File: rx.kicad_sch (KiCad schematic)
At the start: 1 part, among them U1 CC1200

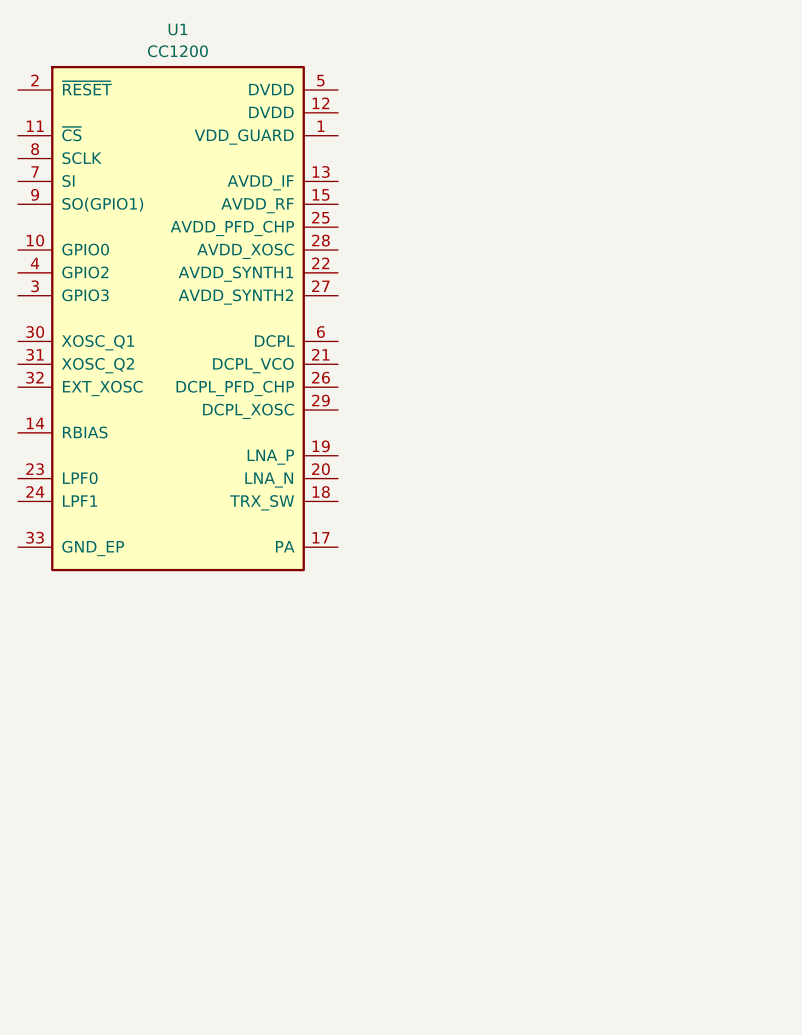
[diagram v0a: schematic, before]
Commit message: Add files via upload
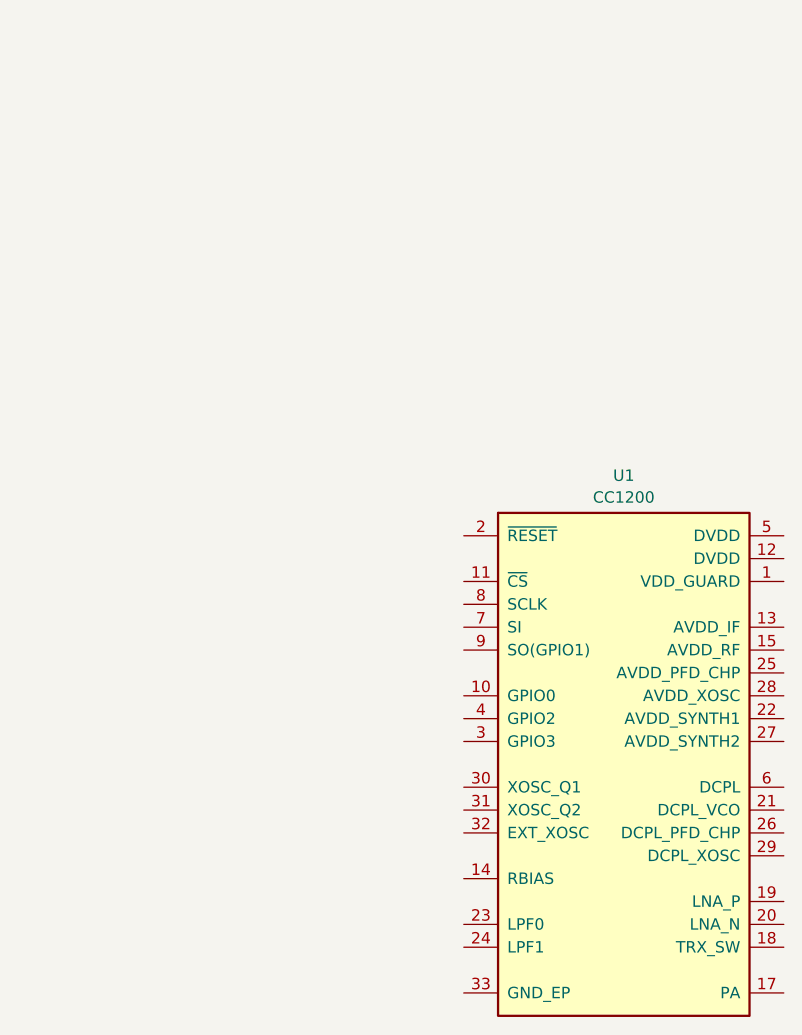
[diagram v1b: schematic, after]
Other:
- moved on the sheet: U1
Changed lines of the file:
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@@
     (comment 1 "Wojciech Kaczmarski, SP5WWP")
   )
-  (symbol (lib_id "RF:CC1200") (at 140.97 91.44 0) (unit 1)
+  (symbol (lib_id "RF:CC1200") (at 190.5 140.97 0) (unit 1)
     (in_bom yes) (on_board yes) (dnp no) (fields_autoplaced)
-    (property "Reference" "U1" (at 140.97 59.3557 0)
+    (property "Reference" "U1" (at 190.5 108.8857 0)
       (effects (font (size 1.27 1.27)))
     )
-    (property "Value" "CC1200" (at 140.97 61.7799 0)
+    (property "Value" "CC1200" (at 190.5 111.3099 0)
       (effects (font (size 1.27 1.27)))
     )
-    (property "Footprint" "Package_DFN_QFN:QFN-32-1EP_5x5mm_P0.5mm_EP3.45x3.45mm" (at 156.21 62.23 0)
+    (property "Footprint" "Package_DFN_QFN:QFN-32-1EP_5x5mm_P0.5mm_EP3.45x3.45mm" (at 205.74 111.76 0)
       (effects (font (size 1.27 1.27)) hide)
     )
-    (property "Datasheet" "http://www.ti.com/lit/ds/symlink/cc1200.pdf" (at 128.27 62.23 0)
+    (property "Datasheet" "http://www.ti.com/lit/ds/symlink/cc1200.pdf" (at 177.8 111.76 0)
       (effects (font (size 1.27 1.27)) hide)
     )
@@
         )
         (path "/4c42207c-9e6b-42da-ad38-da126b892014/67f0dbce-cbd0-480e-94dd-fb4f6a57e3e4"
-          (reference "U9") (unit 1)
+          (reference "U10") (unit 1)
         )
       )

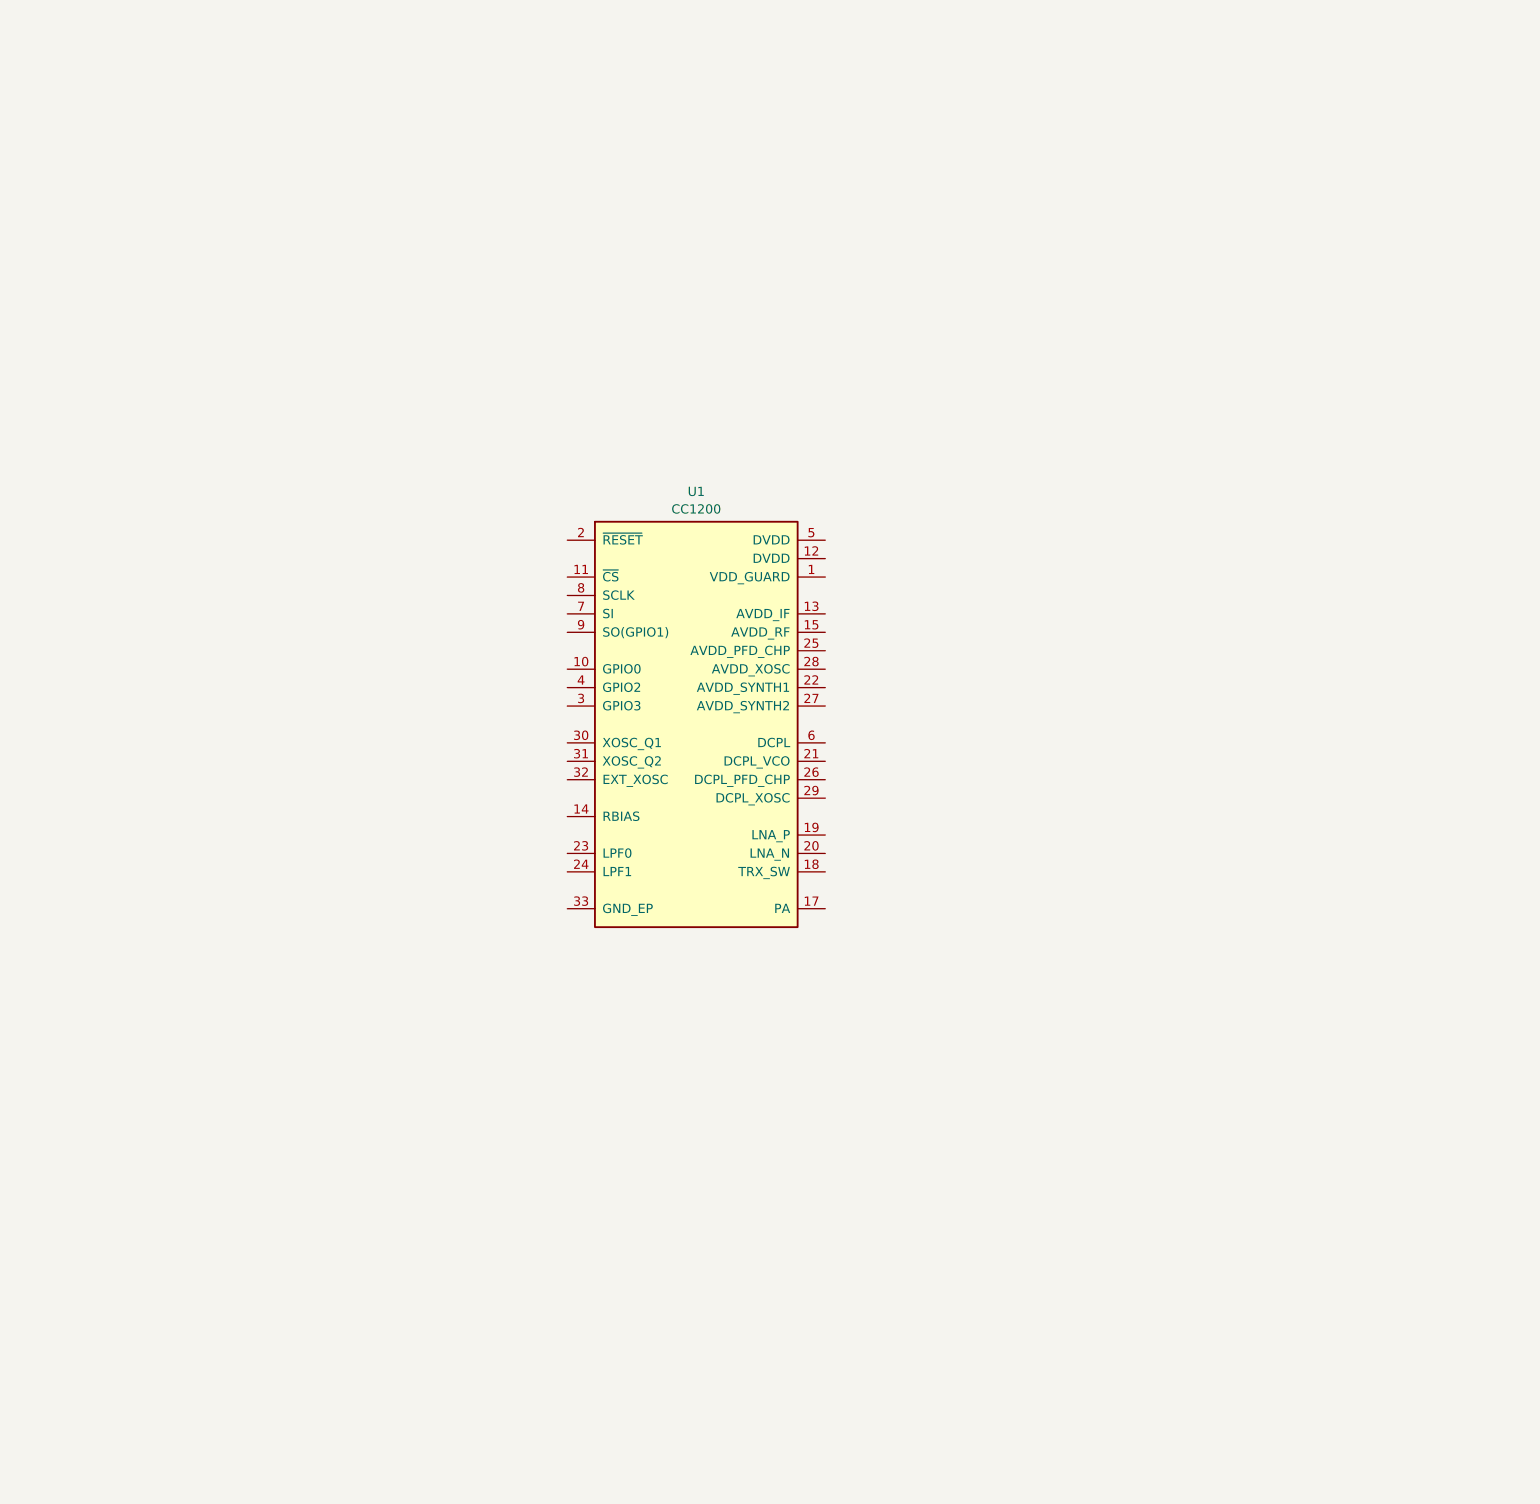
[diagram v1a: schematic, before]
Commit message: Add files via upload
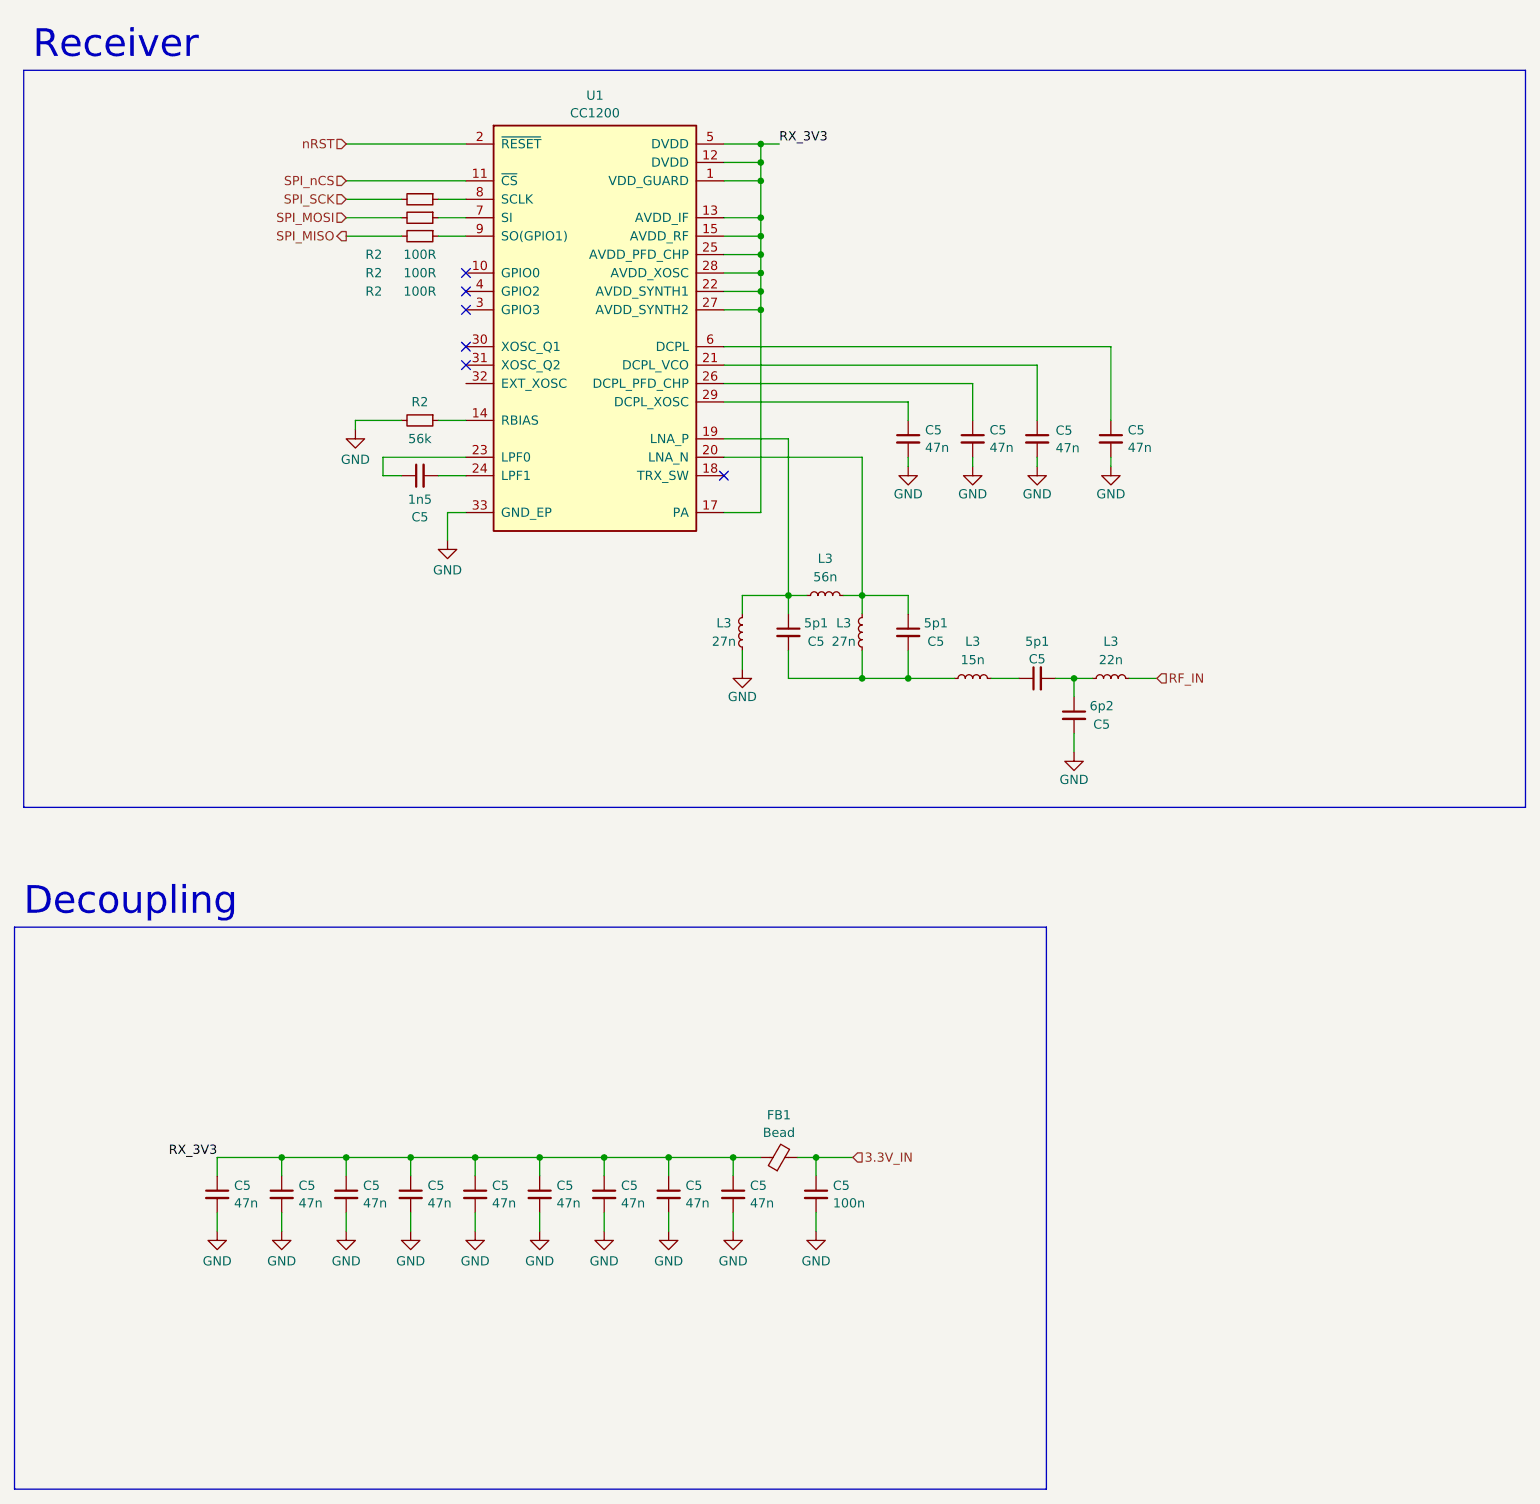
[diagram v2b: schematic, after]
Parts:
- added C5 (x13): 47n, Capacitor_SMD:C_0603_1608Metric, symbol Device:C_Small
- added C5: 1n5, Capacitor_SMD:C_0603_1608Metric, symbol Device:C_Small
- added C5 (x3): 5p1, Capacitor_SMD:C_0603_1608Metric, symbol Device:C_Small
- added C5: 100n, Capacitor_SMD:C_0603_1608Metric, symbol Device:C_Small
- added C5: 6p2, Capacitor_SMD:C_0603_1608Metric, symbol Device:C_Small
- added FB1: Bead, Inductor_SMD:L_0603_1608Metric, symbol Device:FerriteBead_Small
- added L3: 15n, Inductor_SMD:L_0603_1608Metric, symbol Device:L_Small
- added L3 (x2): 27n, Inductor_SMD:L_0603_1608Metric, symbol Device:L_Small
- added L3: 22n, Inductor_SMD:L_0603_1608Metric, symbol Device:L_Small
- added L3: 56n, Inductor_SMD:L_0603_1608Metric, symbol Device:L_Small
- added R2 (x3): 100R, Resistor_SMD:R_0603_1608Metric, symbol Device:R_Small
- added R2: 56k, Resistor_SMD:R_0603_1608Metric, symbol Device:R_Small
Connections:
- net RX_3V3: now reaches U1.1 (VDD_GUARD)
- net RX_3V3: now also U1.12 (DVDD), U1.13 (AVDD_IF), U1.15 (AVDD_RF), U1.17 (PA), U1.22 (AVDD_SYNTH1), U1.25 (AVDD_PFD_CHP), U1.27 (AVDD_SYNTH2), U1.28 (AVDD_XOSC), U1.5 (DVDD), C5.1, C5.1, C5.1, C5.1, C5.1, C5.1, C5.1, C5.1, C5.1, FB1.1
- net SPI_nCS: now reaches U1.11 (~{CS})
- net at U1.14 (RBIAS): now also R2.1
- net at U1.19 (LNA_P): now also C5.1, L3.1, L3.2
- net nRST: now reaches U1.2 (~{RESET})
- net at U1.20 (LNA_N): now also C5.1, L3.1, L3.1
- net at U1.21 (DCPL_VCO): now also C5.1
- net at U1.23 (LPF0): now also C5.1
- net at U1.24 (LPF1): now also C5.2
- net at U1.26 (DCPL_PFD_CHP): now also C5.1
- net at U1.29 (DCPL_XOSC): now also C5.1
- net GND: now reaches U1.33 (GND_EP)
- net GND: now also C5.2, C5.2, C5.2, C5.2, C5.2, C5.2, C5.2, C5.2, C5.2, C5.2, C5.2, C5.2, C5.2, C5.2, C5.2, L3.2, R2.2
- net at U1.6 (DCPL): now also C5.1
- net at U1.7 (SI): now also R2.1
- net at U1.8 (SCLK): now also R2.1
- net at U1.9 (SO(GPIO1)): now also R2.1
- new net: C5.1, L3.1
- new net: C5.2, C5.2, L3.2, L3.2
- new net: C5.1, C5.2, L3.2
- new net 3.3V_IN: C5.1, FB1.2
- new net RF_IN: L3.1
- new net SPI_MISO: R2.2
- new net SPI_MOSI: R2.2
- new net SPI_SCK: R2.2
- no-connect marks 0 -> 6
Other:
- note added: "Decoupling"
- note added: "Receiver"
- moved on the sheet: U1
